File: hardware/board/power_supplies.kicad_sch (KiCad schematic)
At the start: 42 parts, among them J4 Barrel_Jack_Switch, U2 LP2985-3.3, U6 LM27762, U8 LT3506

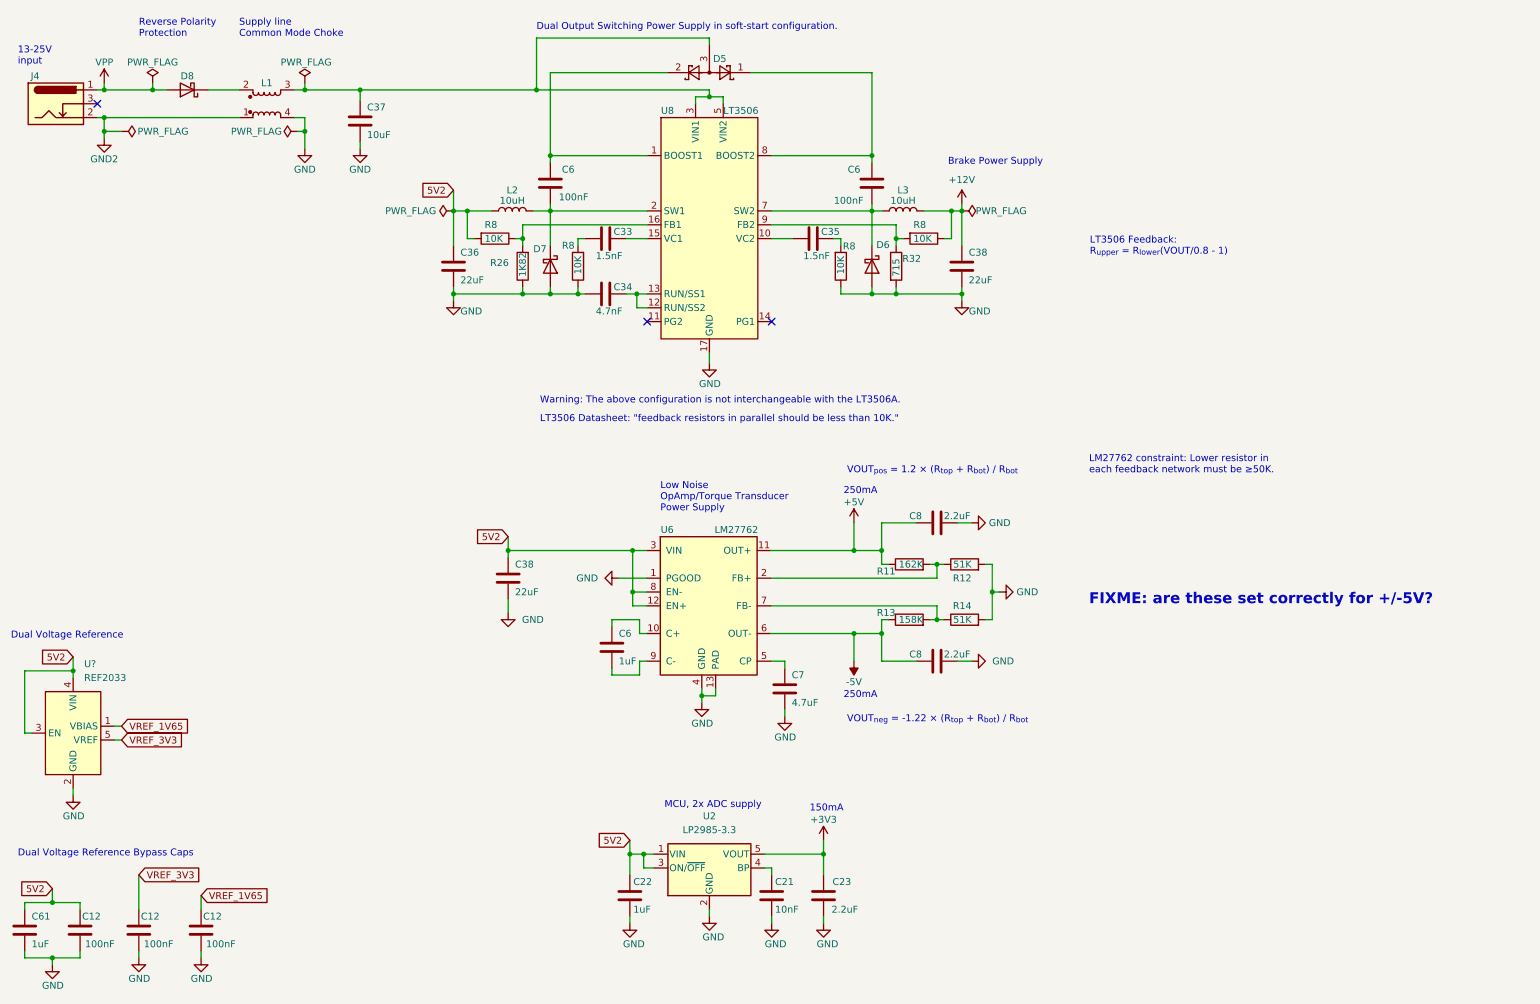
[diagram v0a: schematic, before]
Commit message: update schematic; continue pcb draft
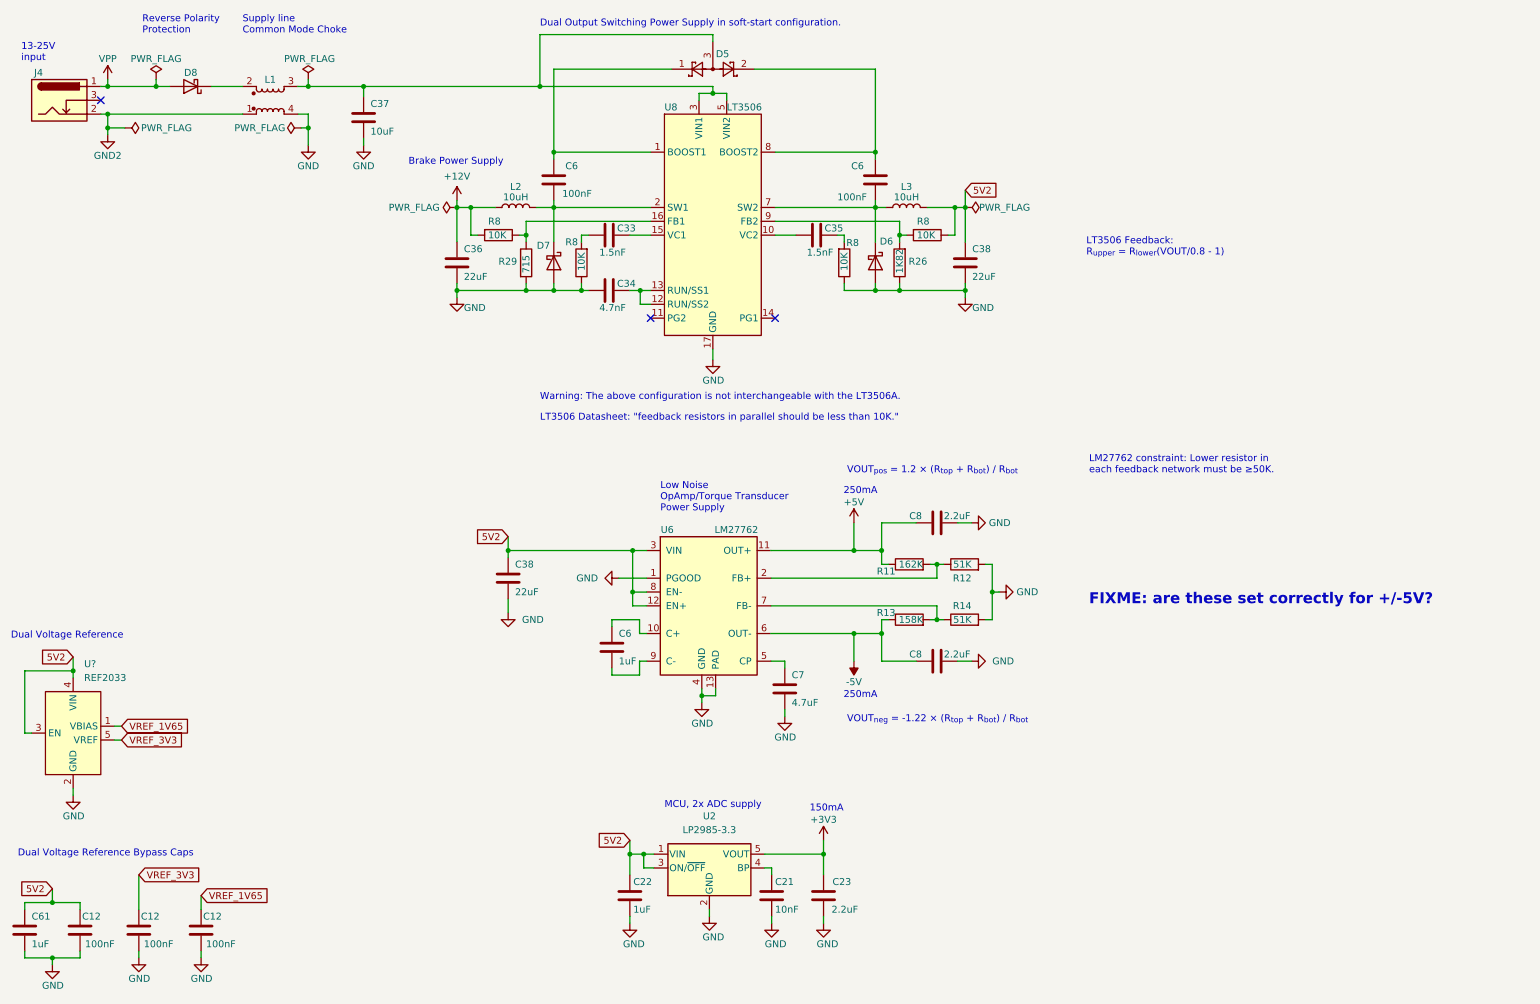
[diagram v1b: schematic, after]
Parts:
- R8: Notes DNP -> (none)
- renumbered R32 to R29
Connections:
- net +12V: now also C36.1, L2.1, R8.2; no longer C38.1, L3.2, R8.1
- net 5V2: now also C38.1, L3.2, R8.1; no longer C36.1, L2.1, R8.2
- net at C6.2, U8.8 (BOOST2): now also D5.2; no longer D5.1
- net at C6.2, U8.1 (BOOST1): now also D5.1; no longer D5.2
- net at R8.1, U8.16 (FB1): now also R29.1; no longer R26.2
- net at R8.2, U8.9 (FB2): now also R26.2; no longer R29.1
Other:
- moved on the sheet: C33, C34, C35, C36, C37, C38, C6, D5, D6, D7, D8, J4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
